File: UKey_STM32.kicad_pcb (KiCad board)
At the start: 2 copper layers, 40.4 x 26.2 mm, 22 parts, among them J1 USB_A, J2 Conn_01x04_Male, SW1 SW_Push, SW2 SW_DIP_x02, U1 NUF2221W1, U2 LDK130-33_SOT23_SOT353, U3 M25PX32-VMW, U4 STM32F103C8Tx, Y1 Crystal_GND24

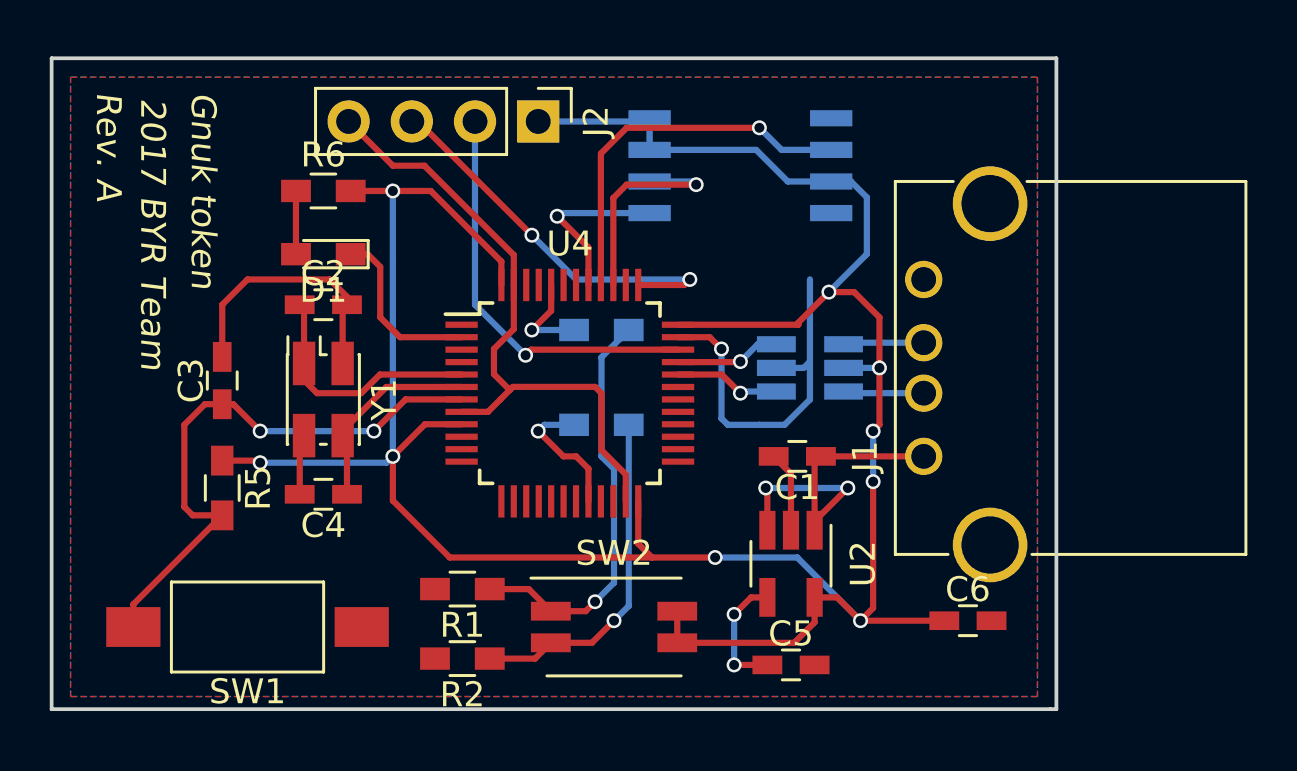
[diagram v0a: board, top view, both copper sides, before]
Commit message: Updated board.
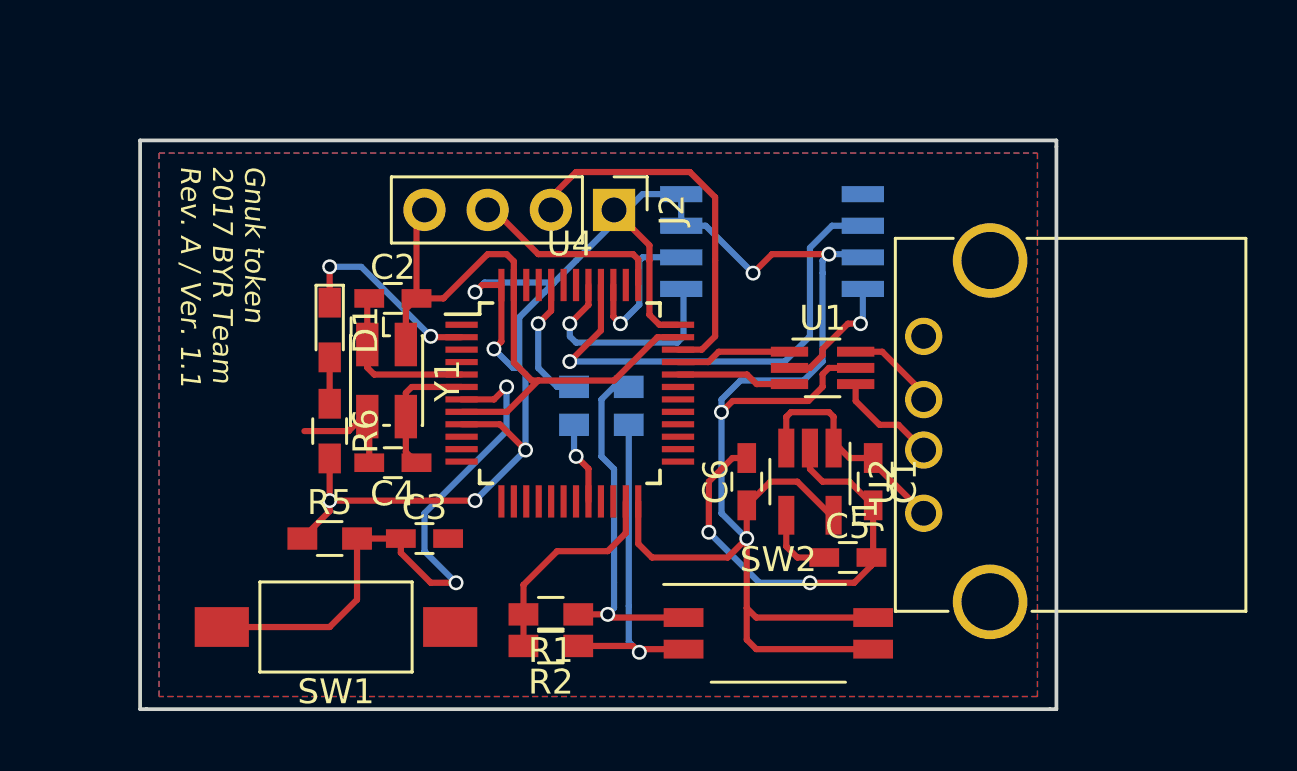
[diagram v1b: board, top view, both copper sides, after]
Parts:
- SW2: footprint Buttons_Switches_SMD:SW_DIP_x2_W5.08mm_Slide_Copal_CHS-A -> Buttons_Switches_SMD:SW_DIP_x2_W7.62mm_Slide_Copal_CHS-B
- U1: footprint TO_SOT_Packages_SMD:SOT-23-6_Handsoldering -> TO_SOT_Packages_SMD:SOT-363_SC-70-6_Handsoldering; moved to F.Cu
- moved C6 10.5 mm to (192.3, 62.2), turned to 90 degrees
- moved C3 10.3 mm to (179.3, 64.5), turned to 0 degrees
- moved R6 9.66 mm to (175.5, 60.2), turned to 270 degrees
- moved SW2 6.61 mm to (193.5, 68.3)
- moved C5 4.89 mm to (196.3, 65.3)
- moved R5 4.77 mm to (175.5, 64.5), turned to 0 degrees
- moved J2 4.68 mm to (186.9, 51.3)
- moved R1 3.70 mm to (184.4, 67.6)
- moved R2 3.59 mm to (184.4, 68.8)
- moved SW1 3.56 mm to (175.8, 68.1)
- moved U2 3.39 mm to (194.8, 62.2)
- moved U3 3.30 mm to (193.3, 52.6)
- moved C1 3.21 mm to (197.4, 62.2), turned to 270 degrees
- moved C4 3.07 mm to (178.1, 61.5)
- moved D1 3.06 mm to (175.5, 56.1), turned to 270 degrees
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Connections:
- U1 pad 1: USB_DM -> USB_DP
- U1 pad 3: USB_DP -> USB_DM
- U1 pad 4: EMI_DP -> EMI_DM
- U1 pad 6: EMI_DM -> EMI_DP
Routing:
- net VCC: track 111.4 -> 102.6 mm
- net SWCLK: track 16.0 -> 7.90 mm, vias 2 -> 0
- net VBUS: track 14.5 -> 9.45 mm, vias 2 -> 0
- net HSE_IN: track 11.0 -> 6.72 mm
- net SPI_MISO: track 15.5 -> 19.7 mm
- net GND: track 58.2 -> 62.4 mm, vias 1 -> 3
- net HSE_OUT: track 8.14 -> 5.32 mm
- net SPI_SCK: track 8.97 -> 6.27 mm
- net BOOT1: track 5.51 -> 3.32 mm
- net Net-(R1-Pad1): track 16.7 -> 14.5 mm
- net SPI_MOSI: track 7.05 -> 9.10 mm
- net Net-(C5-Pad1): track 4.99 -> 2.96 mm, vias 2 -> 0
- net NRST: track 23.4 -> 25.2 mm
- net BOOT0: track 3.82 -> 5.31 mm
- net SWDIO: track 16.5 -> 15.3 mm, vias 1 -> 0
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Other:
- board size 40.4 x 26.2 mm -> 36.8 x 22.9 mm
- board text added: "Gnuk token 2017 BYR Team Rev. A / Ver. 1.1"
- board text removed: "2017 BYR Team"
- board text removed: "Gnuk token"
- board text removed: "Rev. A"
